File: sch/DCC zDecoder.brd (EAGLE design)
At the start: 100 x 80 mm, 25 parts, among them IC1 5V, IC2 ULN2803, IC3 ULN2803, X10 22-23-2031, X11 22-23-2031, X12 22-23-2031, X7 22-23-2031, X8 22-23-2031, X9 22-23-2031

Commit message: partlist updated
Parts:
- B1: value (none) -> B80R DIO
- ESP1: value (none) -> ESP32 NodeMCU
- IC1: value 5V -> TSR 1-2450
- J1: value (none) -> MPE 087-1-003
- LED1: value green -> green 3mm
- RESET: value (none) -> MPE 087-1-002
- X1, X2, X3, X4: value (none) -> DG240 2,54-8
- X10, X11, X12, X7, X8, X9: value 22-23-2031 -> PSS 254/3G
- X5, X6: value (none) -> DG240 2,54-2

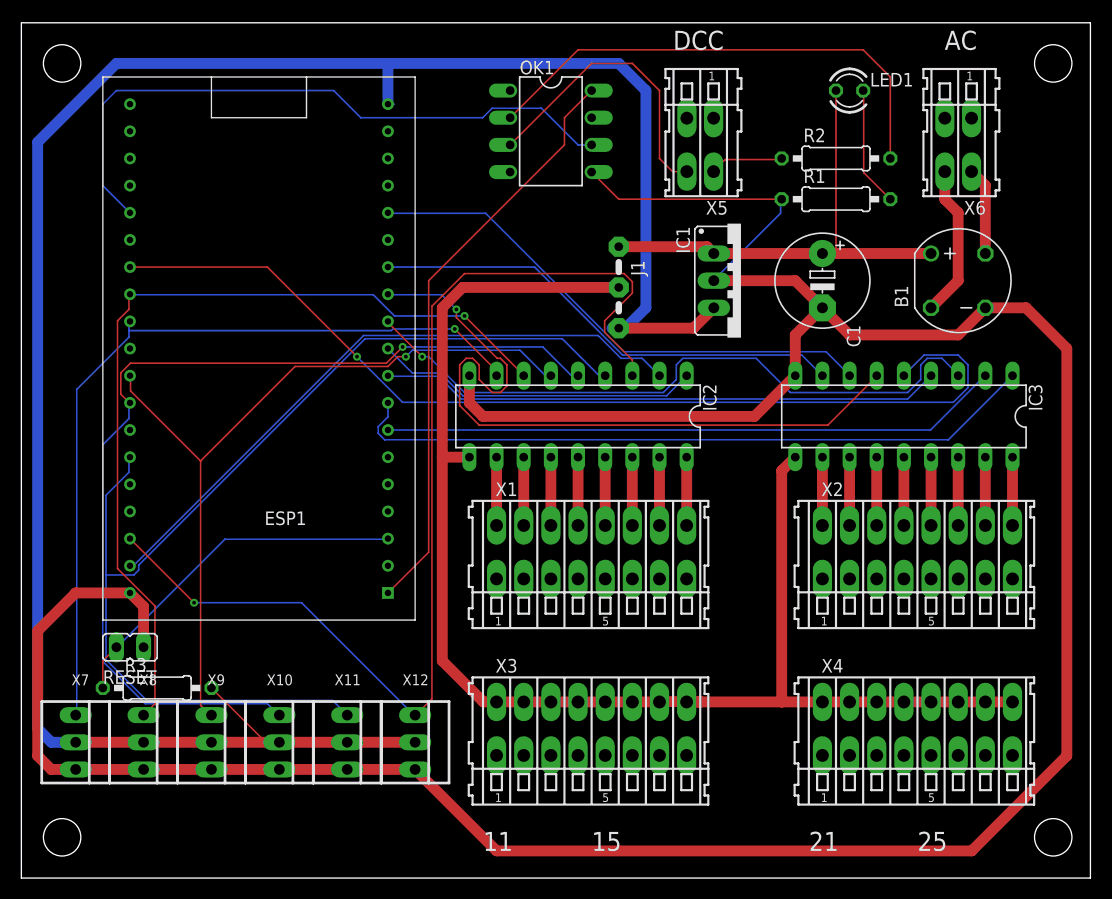
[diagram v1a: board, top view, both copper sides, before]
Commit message: backup
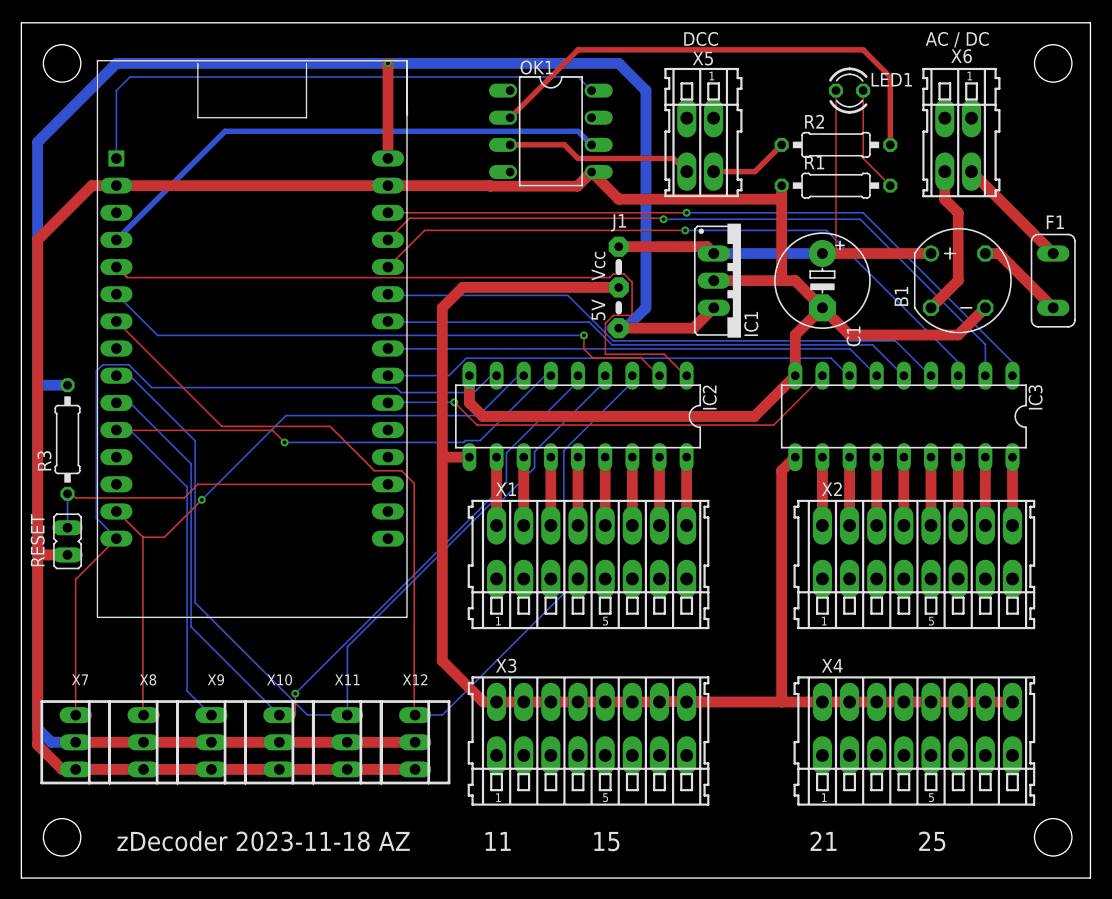
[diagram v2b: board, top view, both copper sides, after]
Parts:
- added F1: 900mA, fuse:TE5
- ESP1: value ESP32 NodeMCU -> NodeMCU CH340C; device _esp32:ESP32_NODEMCU -> _esp32:ESP32_NODEMCU_CH340C
- moved ESP1 25.7 mm to (8.89, 63.5)
- moved R3 24.7 mm to (4.32, 41.0), turned to 90 degrees
- moved RESET 11.5 mm to (4.32, 31.5), turned to 180 degrees
- moved R1 1.27 mm to (76.2, 64.8)
- moved R2 1.27 mm to (76.2, 68.6)
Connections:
- removed net GND1: ESP1.14
- removed net GND2: ESP1.32
- new net N$15: F1.1, X6.A1
- net +3V3: now also ESP1.P$1; no longer ESP1.1
- net +5V: now also ESP1.P$30; no longer ESP1.19
- net GND: now also ESP1.P$2, ESP1.P$29; no longer ESP1.38
- net GPIO2: now also ESP1.P$4; no longer ESP1.24
- net GPIO39: now also ESP1.P$18; no longer ESP1.3
- net N$5: now also F1.2; no longer X6.A1
- net O11: now also ESP1.P$15; no longer ESP1.28
- net O12: now also ESP1.P$14; no longer ESP1.27
- net O13: now also ESP1.P$11; no longer ESP1.30
- net O14: now also ESP1.P$10; no longer ESP1.31
- net O15: now also ESP1.P$9; no longer ESP1.33
- net O16: now also ESP1.P$7; no longer ESP1.36
- net O17: now also ESP1.P$6; no longer ESP1.37
- net O18: now also ESP1.P$5; no longer ESP1.10
- net O21: now also ESP1.P$21; no longer ESP1.13
- net O22: now also ESP1.P$22; no longer ESP1.15
- net O23: now also ESP1.P$23; no longer ESP1.12
- net O24: now also ESP1.P$24; no longer ESP1.26
- net O25: now also ESP1.P$25; no longer ESP1.9
- net O26: now also ESP1.P$26; no longer ESP1.11
- net O27: now also ESP1.P$27; no longer ESP1.7
- net O28: now also ESP1.P$28; no longer ESP1.8
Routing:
- net O24: track 93.5 -> 50.4 mm, vias 1 -> 0
- net GND: track 280.7 -> 240.6 mm
- net O18: track 30.5 -> 67.7 mm
- net O23: track 68.9 -> 46.8 mm, vias 1 -> 0
- net O12: track 81.8 -> 62.0 mm
- net O15: track 102.2 -> 86.0 mm
- net O14: track 91.9 -> 80.4 mm
- net GPIO2: track 60.3 -> 49.2 mm
- net N$15: track 0.00 -> 10.8 mm
- net N$11: track 27.6 -> 17.6 mm
- net O27: track 58.0 -> 64.6 mm, vias 0 -> 1
- net O16: track 103.7 -> 97.5 mm, vias 1 -> 0
- net O22: track 49.5 -> 44.5 mm
- net O17: track 60.0 -> 55.0 mm, vias 0 -> 1
- net +3V3: track 54.9 -> 51.9 mm
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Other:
- board text added: "5V"
- board text added: "AC / DC"
- board text added: "Vcc"
- board text added: "zDecoder 2023-11-18 AZ"
- board text removed: "AC"
